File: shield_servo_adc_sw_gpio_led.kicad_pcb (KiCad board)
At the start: 2 copper layers, 70 x 40 mm, 42 parts, among them J1 srv,adc, J10 Conn_02x01, J2 srv,adc, J3 srv,adc, J4 srv,adc, J5 srv,adc, J6 srv,adc, J7 srv,adc, J8 srv,adc, J9 usart,i2c, U1 moricleo

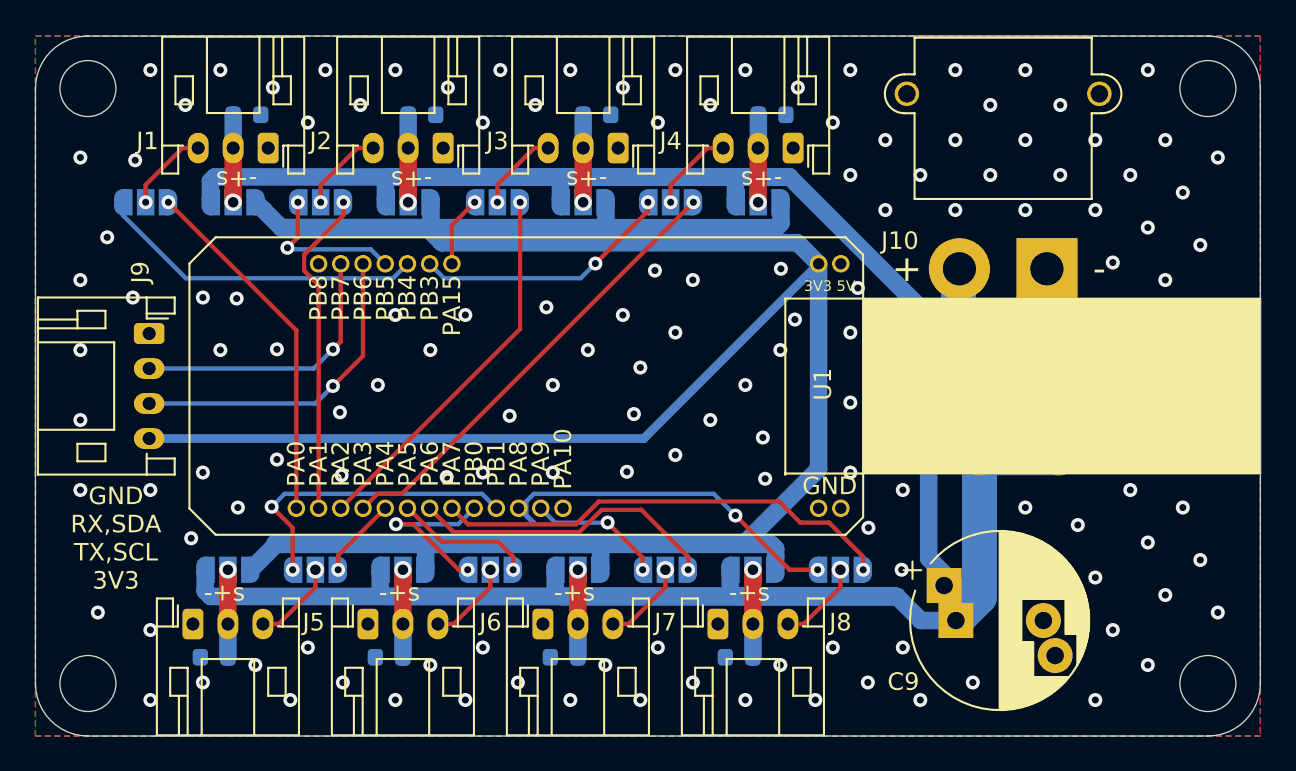
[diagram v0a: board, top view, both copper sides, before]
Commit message: solenoid 完成
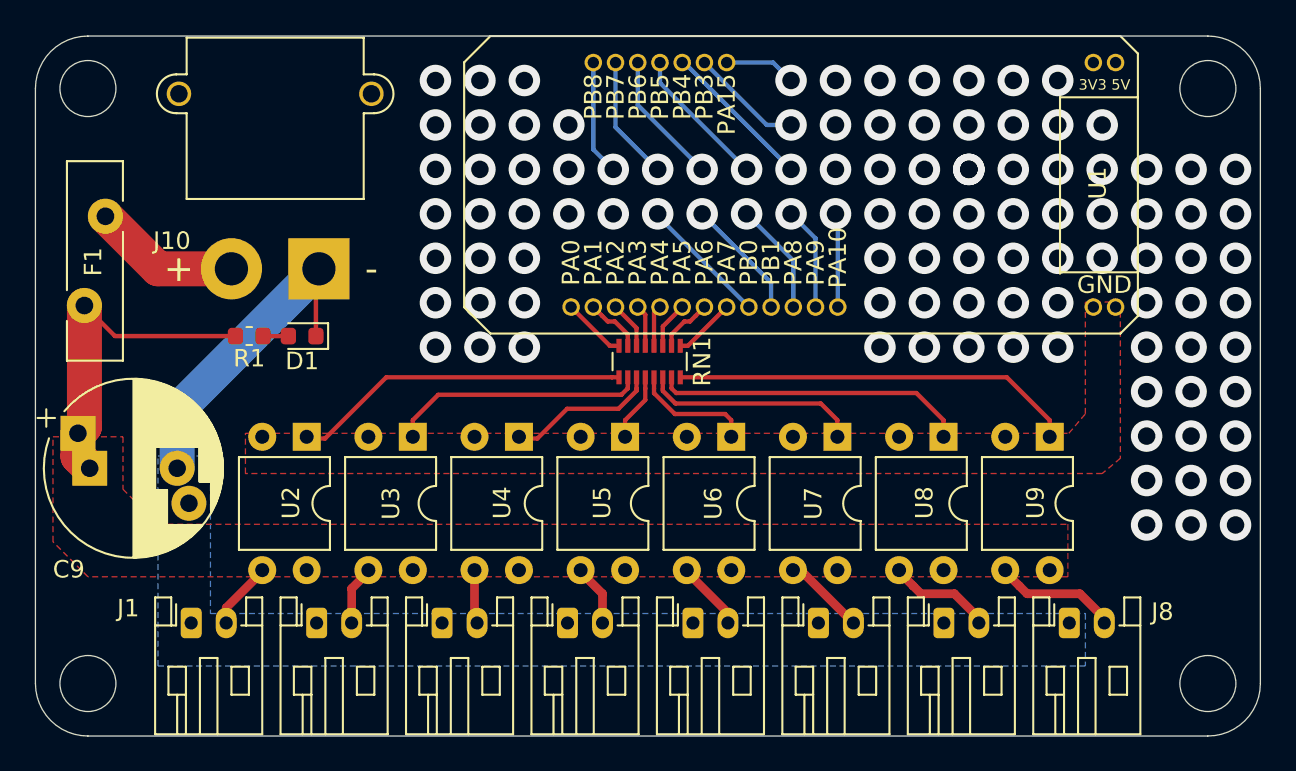
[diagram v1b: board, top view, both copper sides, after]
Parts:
- removed C1, C2, C3, C4, C5, C6, C7, C8: 1u, Capacitor_SMD:C_0603_1608Metric
- removed F2: 30V6A, Fuse:Fuse_Bourns_MF-RHT600
- removed J9: usart,i2c, Connector_JST:JST_PH_S4B-PH-K_1x04_P2.00mm_Horizontal
- removed JP1, JP10, JP11, JP12, JP13, JP14, JP15, JP16, JP2, JP3, JP4, JP5, JP6, JP7, JP8, JP9: jumper, Jumper:SolderJumper-3_P1.3mm_Open_RoundedPad1.0x1.5mm_NumberLabels
- added D1: LED, LED_SMD:LED_0603_1608Metric, F.Cu at (205.2, 136.1)
- added R1: R, Resistor_SMD:R_0603_1608Metric, F.Cu at (202.2, 136.1)
- added RN1: R_Pack08, Resistor_SMD:R_Array_Convex_8x0602, F.Cu at (225.1, 137.6)
- added U2: TLP627, Package_DIP:DIP-4_W7.62mm, F.Cu at (205.5, 141.9)
- added U3: TLP627, Package_DIP:DIP-4_W7.62mm, F.Cu at (211.6, 141.9)
- added U4: TLP627, Package_DIP:DIP-4_W7.62mm, F.Cu at (217.6, 141.9)
- added U5: TLP627, Package_DIP:DIP-4_W7.62mm, F.Cu at (223.7, 141.9)
- added U6: TLP627, Package_DIP:DIP-4_W7.62mm, F.Cu at (229.8, 141.9)
- added U7: TLP627, Package_DIP:DIP-4_W7.62mm, F.Cu at (235.8, 141.9)
- added U8: TLP627, Package_DIP:DIP-4_W7.62mm, F.Cu at (241.9, 141.9)
- added U9: TLP627, Package_DIP:DIP-4_W7.62mm, F.Cu at (248.0, 141.9)
- F1: moved to F.Cu
- J1, J2, J3, J4, J5, J6, J7, J8: value srv,adc -> Solenoid; footprint Connector_JST:JST_PH_S3B-PH-K_1x03_P2.00mm_Horizontal -> Connector_JST:JST_PH_S2B-PH-K_1x02_P2.00mm_Horizontal
- moved F1 56.4 mm to (192.8, 134.4)
- moved C9 50.3 mm to (193.1, 143.7)
- moved J10 41.6 mm to (206.2, 132.3)
- moved J4 30.0 mm to (220.4, 152.5), turned to 0 degrees
- moved J3 28.9 mm to (213.2, 152.5), turned to 0 degrees
- moved J5 28.6 mm to (227.6, 152.5)
- moved J2 28.1 mm to (206.1, 152.5), turned to 0 degrees
- moved J1 27.5 mm to (198.9, 152.5), turned to 0 degrees
- moved J6 25.7 mm to (234.7, 152.5)
- moved J7 22.9 mm to (241.9, 152.5)
- moved J8 20.1 mm to (249.1, 152.5)
- moved U1 19.5 mm to (229.5, 127.5)
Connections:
- C9 pad 2: GND -> GNDPWR
- J1 pad 1: GND -> GNDPWR
- J10 pad 1: GND -> GNDPWR
- J2 pad 1: GND -> GNDPWR
- J3 pad 1: GND -> GNDPWR
- J4 pad 1: GND -> GNDPWR
- J5 pad 1: GND -> GNDPWR
- J6 pad 1: GND -> GNDPWR
- J7 pad 1: GND -> GNDPWR
- J8 pad 1: GND -> GNDPWR
- U1 pad 10: /PWM4 -> Net-(U1-Pad10)
- U1 pad 11: /PWM7 -> Net-(U1-Pad11)
- U1 pad 12: /PWM6 -> Net-(U1-Pad12)
- U1 pad 13: (no net) -> Net-(U1-Pad13)
- U1 pad 14: /PWM2 -> Net-(U1-Pad14)
- U1 pad 15: /PWM3 -> Net-(U1-Pad15)
- U1 pad 16: /PWM0 -> Net-(U1-Pad16)
- U1 pad 17: /PWM1 -> Net-(U1-Pad17)
- U1 pad 18: /TX,SCL -> Net-(U1-Pad18)
- U1 pad 19: /RX,SDA -> Net-(U1-Pad19)
- U1 pad 20: (no net) -> Net-(U1-Pad20)
- U1 pad 21: +3V3 -> Net-(U1-Pad21)
- U1 pad 22: (no net) -> Net-(U1-Pad22)
- U1 pad 9: /PWM5 -> Net-(U1-Pad9)
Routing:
- net +3V3: track 233.6 -> 0.00 mm
- net VCC: track 228.7 -> 19.1 mm
- net /AD3: track 26.1 -> 2.39 mm, vias 1 -> 0
- net Net-(RN1-Pad16): track 0.00 -> 23.2 mm
- net /AD7: track 26.5 -> 3.57 mm, vias 1 -> 0
- net /PWM7: track 21.2 -> 0.00 mm, vias 2 -> 0
- net Net-(RN1-Pad9): track 0.00 -> 19.3 mm
- net /AD2: track 21.7 -> 2.71 mm, vias 1 -> 0
- net /PWM0: track 18.8 -> 0.00 mm
- net GNDPWR: track 0.00 -> 18.7 mm
- net /TX,SCL: track 18.6 -> 0.00 mm, vias 1 -> 0
- net Net-(RN1-Pad15): track 0.00 -> 18.0 mm
- net /PWM4: track 17.6 -> 0.00 mm, vias 2 -> 0
- net /AD0: track 20.5 -> 3.66 mm, vias 1 -> 0
- net /RX,SDA: track 16.0 -> 0.00 mm, vias 1 -> 0
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- added copper zone on B.Cu, net GNDPWR
- added copper zone on F.Cu, net VCC
- removed copper zone on B.Cu, net GND
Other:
- board text removed: "-+s"
- board text removed: "GND RX,SDA TX,SCL 3V3"
- board text removed: "V3"
- board text removed: "pa"
- board text removed: "v3"
